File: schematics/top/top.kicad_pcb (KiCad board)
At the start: 2 copper layers, 45.1 x 45.1 mm, 13 parts, among them J1 CLT-108-02-F-D-BE-K-TR, J2 Conn_01x04_Socket

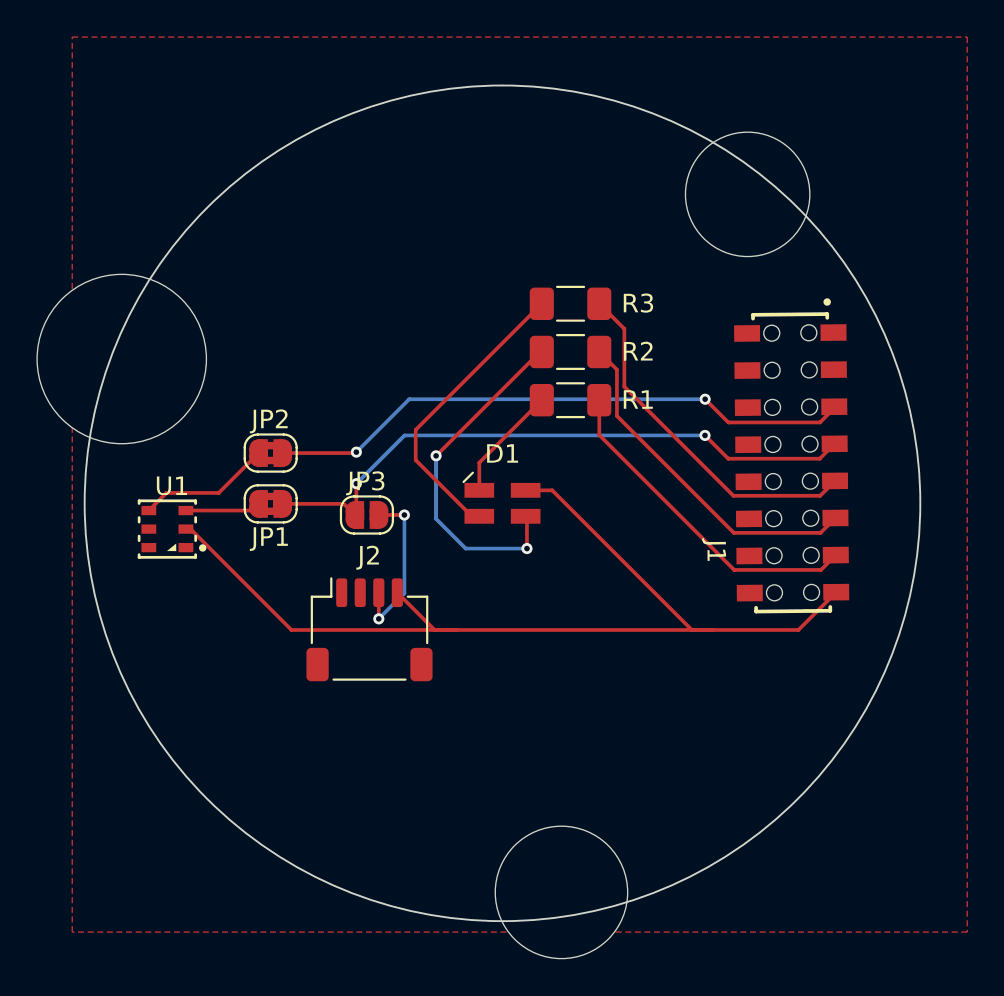
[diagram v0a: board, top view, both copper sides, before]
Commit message: Signed-off-by: Ray33ee <30669752+ray33ee@users.noreply.github.com>
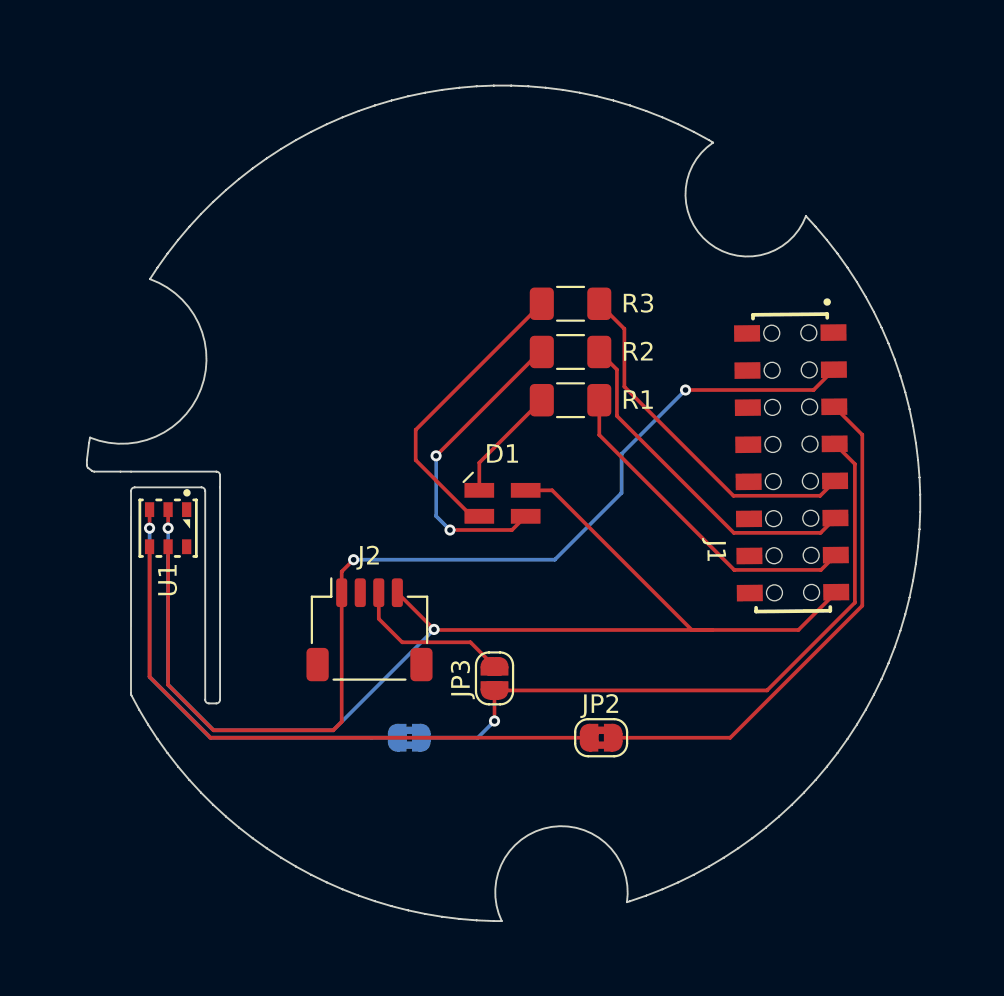
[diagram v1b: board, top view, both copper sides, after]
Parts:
- removed ? (x2): , 
- removed REF**: MountingHole_4mm, MountingHole:MountingHole_4mm
- JP1: moved to B.Cu
- moved JP2 23.5 mm to (143.4, 116.5)
- moved JP1 14.7 mm to (133.1, 116.5)
- moved JP3 11.2 mm to (137.7, 113.3), turned to 90 degrees
- moved U1 0.06 mm to (120.1, 105.2), turned to 90 degrees
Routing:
- net GND: track 0.00 -> 58.4 mm, vias 0 -> 2
- net /SDA: track 7.20 -> 32.1 mm
- net /SCL: track 4.07 -> 23.7 mm, vias 0 -> 1
- net +3V3: track 55.4 -> 65.6 mm, vias 0 -> 2
- net DATA2: track 31.8 -> 27.7 mm, vias 2 -> 0
- net DATA1: track 33.6 -> 36.6 mm, vias 2 -> 1
- net /G: track 18.8 -> 16.8 mm
- net /1WIRE: track 8.95 -> 8.71 mm, vias 2 -> 0
- removed copper zone on F.Cu, net GND
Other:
- board size 45.1 x 45.1 mm -> 44.9 x 45.1 mm
